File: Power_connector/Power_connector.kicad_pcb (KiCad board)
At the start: 2 copper layers, 80.8 x 107.2 mm, 65 parts, among them J1 XT60_F, J10 XT60_F, J11 XT60_F, J12 XT60_F, J13 XT60_F, J14 XT60_F, J2 XT60_Male, J3 XT60_F, J4 E_Stop, J5 XT60_F, J6 XT60_F, J7 XT60_F, J8 XT60_F, J9 XT60_F, Q1 IRFS7530, Q2 IRFS7530

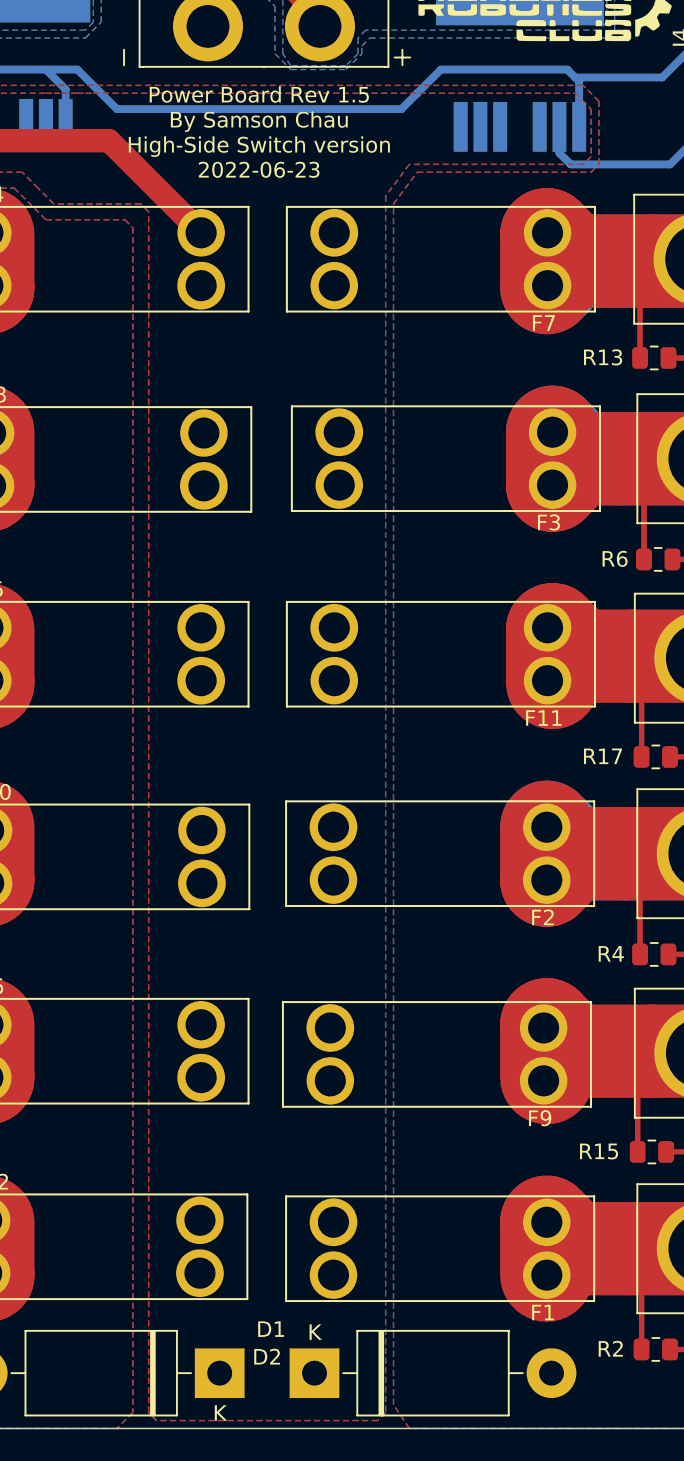
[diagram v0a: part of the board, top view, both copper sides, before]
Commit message: update
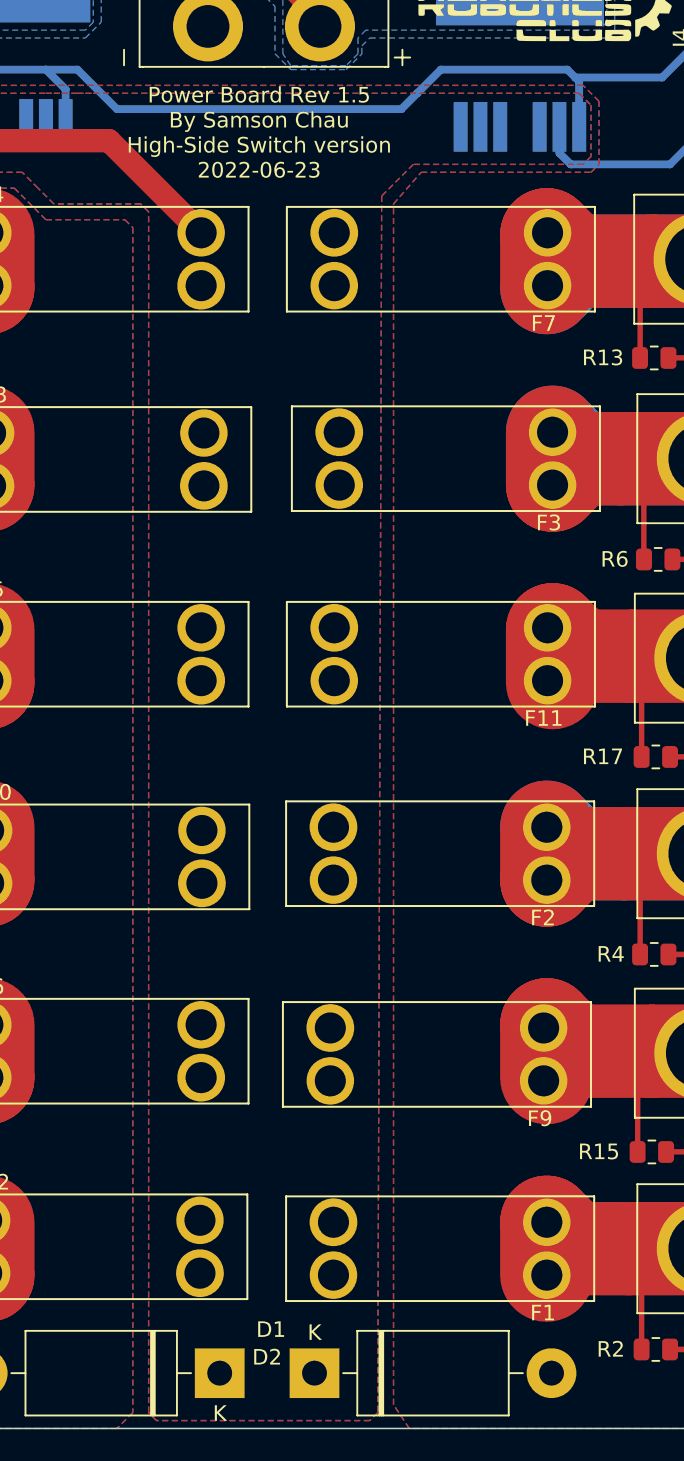
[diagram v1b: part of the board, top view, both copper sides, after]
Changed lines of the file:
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@@
       (pts
         (xy 150.368 66.548)
-        (xy 139.192 66.548)
-        (xy 137.668 68.58)
-        (xy 137.668 146.812)
-        (xy 137.16 147.32)
+        (xy 139.446 66.548)
+        (xy 137.414 68.58)
+        (xy 137.16 146.812)
+        (xy 136.652 147.32)
         (xy 122.936 147.32)
         (xy 122.428 146.812)
@@
         (xy 118.364 61.976)
         (xy 118.872 61.976)
-        (xy 149.86 61.976)
-        (xy 150.876 62.992)
+        (xy 150.114 61.976)
+        (xy 150.876 62.738)
         (xy 150.876 66.04)
       )
@@
         (xy 138.176 146.304)
         (xy 138.176 69.088)
-        (xy 139.7 67.056)
+        (xy 139.954 67.056)
         (xy 150.876 67.056)
         (xy 151.384 66.548)
@@
         (xy 138.176 146.304)
         (xy 138.176 69.088)
-        (xy 139.7 67.056)
+        (xy 139.954 67.056)
         (xy 150.876 67.056)
         (xy 151.384 66.548)
